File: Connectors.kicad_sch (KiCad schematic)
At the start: 8 parts, among them J1 A, J1 A_OUT, J1 B_OUT, J1 C_OUT, J2 B, J3 C, J4 Conn_02x07_Odd_Even, J8 Conn_02x02_Odd_Even

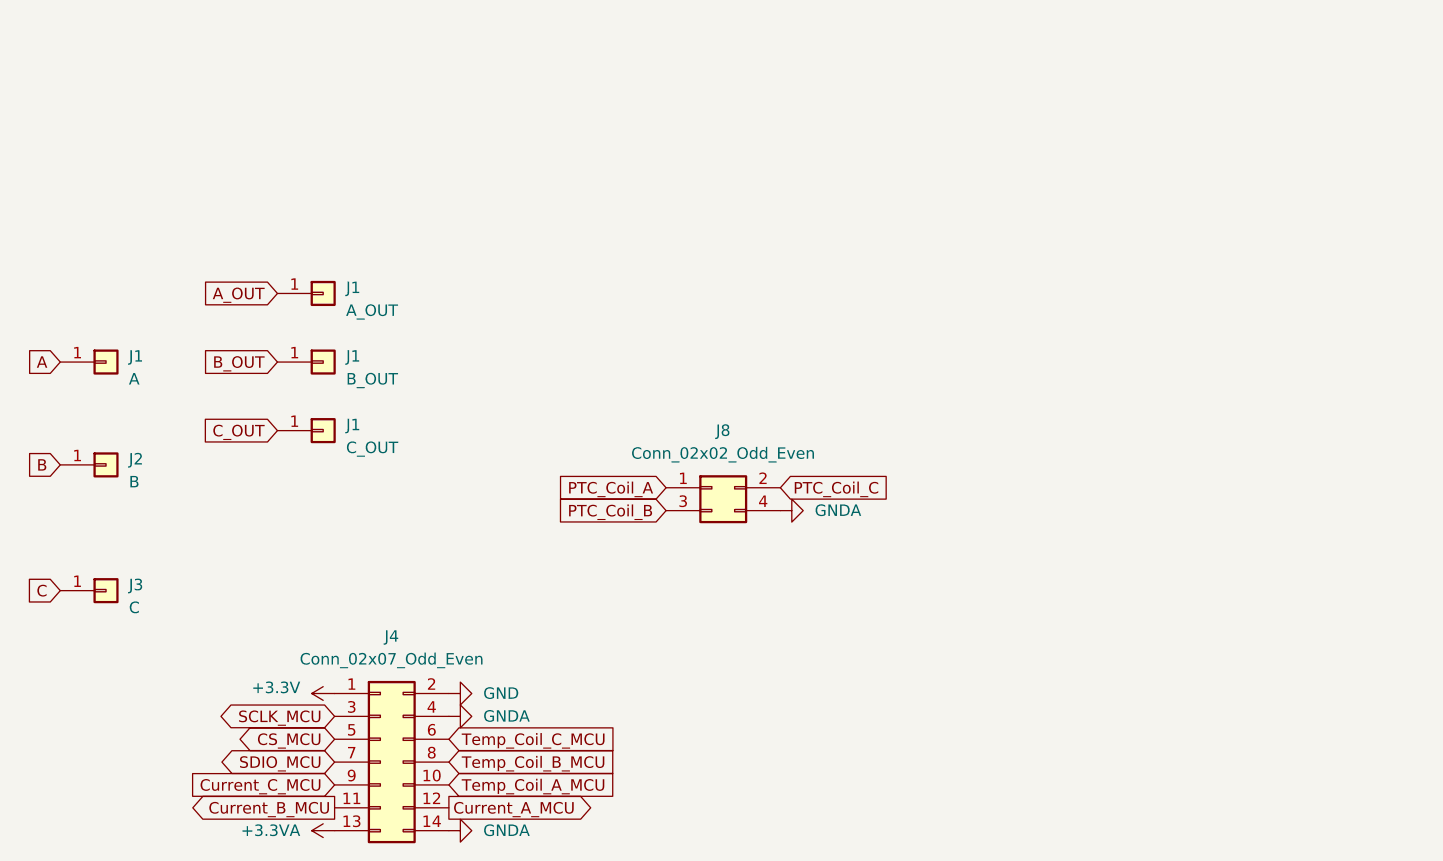
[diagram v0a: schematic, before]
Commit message: С ножевыми разъёмами по кругу
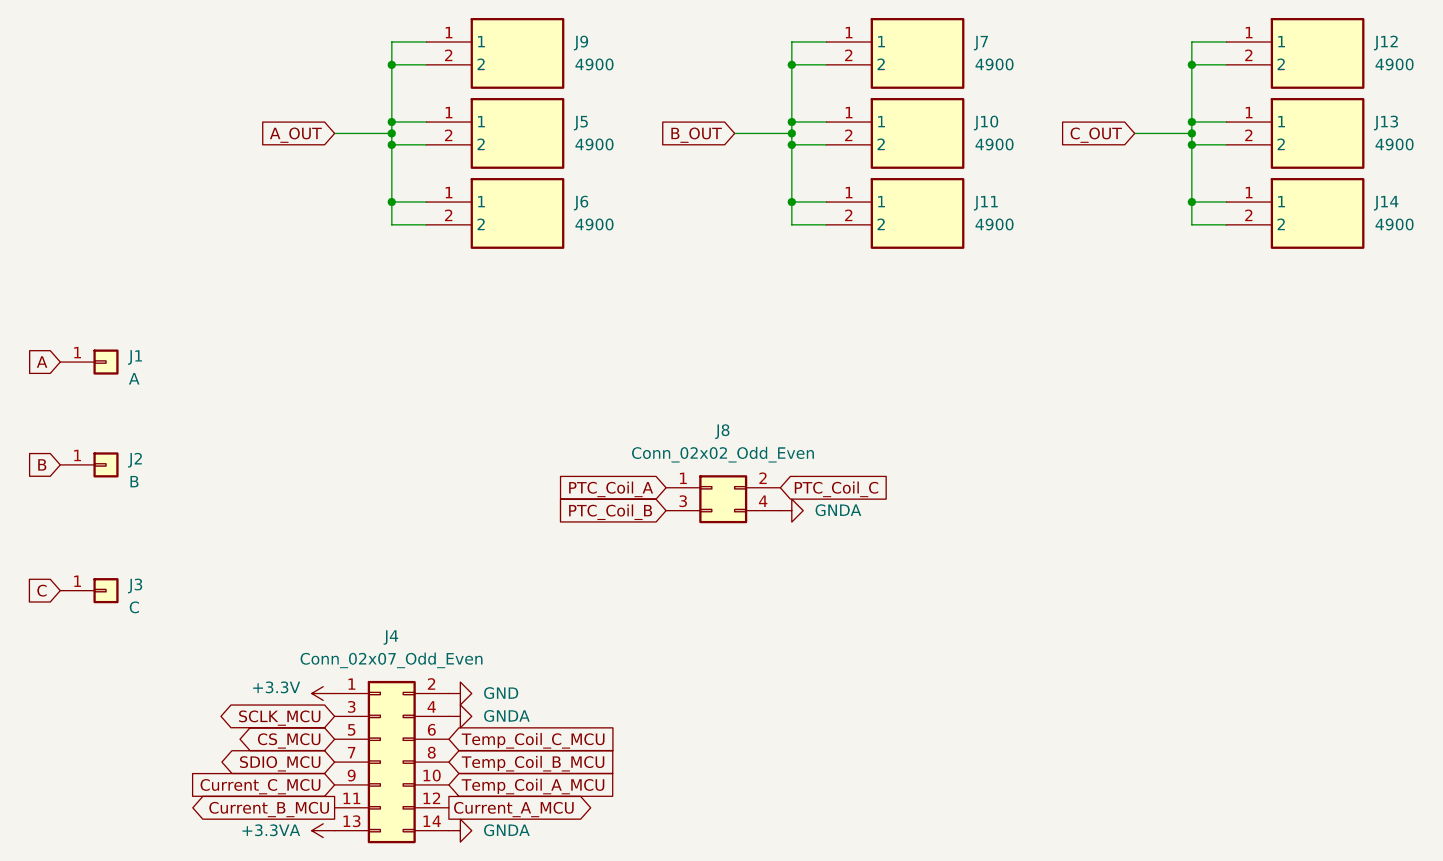
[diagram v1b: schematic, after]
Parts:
- removed J1: A_OUT, Connector_My:Power_Wire, symbol Connector_Generic:Conn_01x01
- removed J1: B_OUT, Connector_My:Power_Wire, symbol Connector_Generic:Conn_01x01
- removed J1: C_OUT, Connector_My:Power_Wire, symbol Connector_Generic:Conn_01x01
- added J10, J11, J12, J13, J14, J5, J6, J7, J9: 4900, Connector_My:4900, symbol 4900:4900
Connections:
- net A_OUT: now also J5.1, J5.2, J6.1, J6.2, J9.1, J9.2
- net B_OUT: now also J10.1, J10.2, J11.1, J11.2, J7.1, J7.2
- net C_OUT: now also J12.1, J12.2, J13.1, J13.2, J14.1, J14.2
